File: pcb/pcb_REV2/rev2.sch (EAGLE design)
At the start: 65 parts, among them IC1 PIC24FJ128GA010, IC2 LM1117-XX, IC3 MAX6520, J1 RJ11-6X

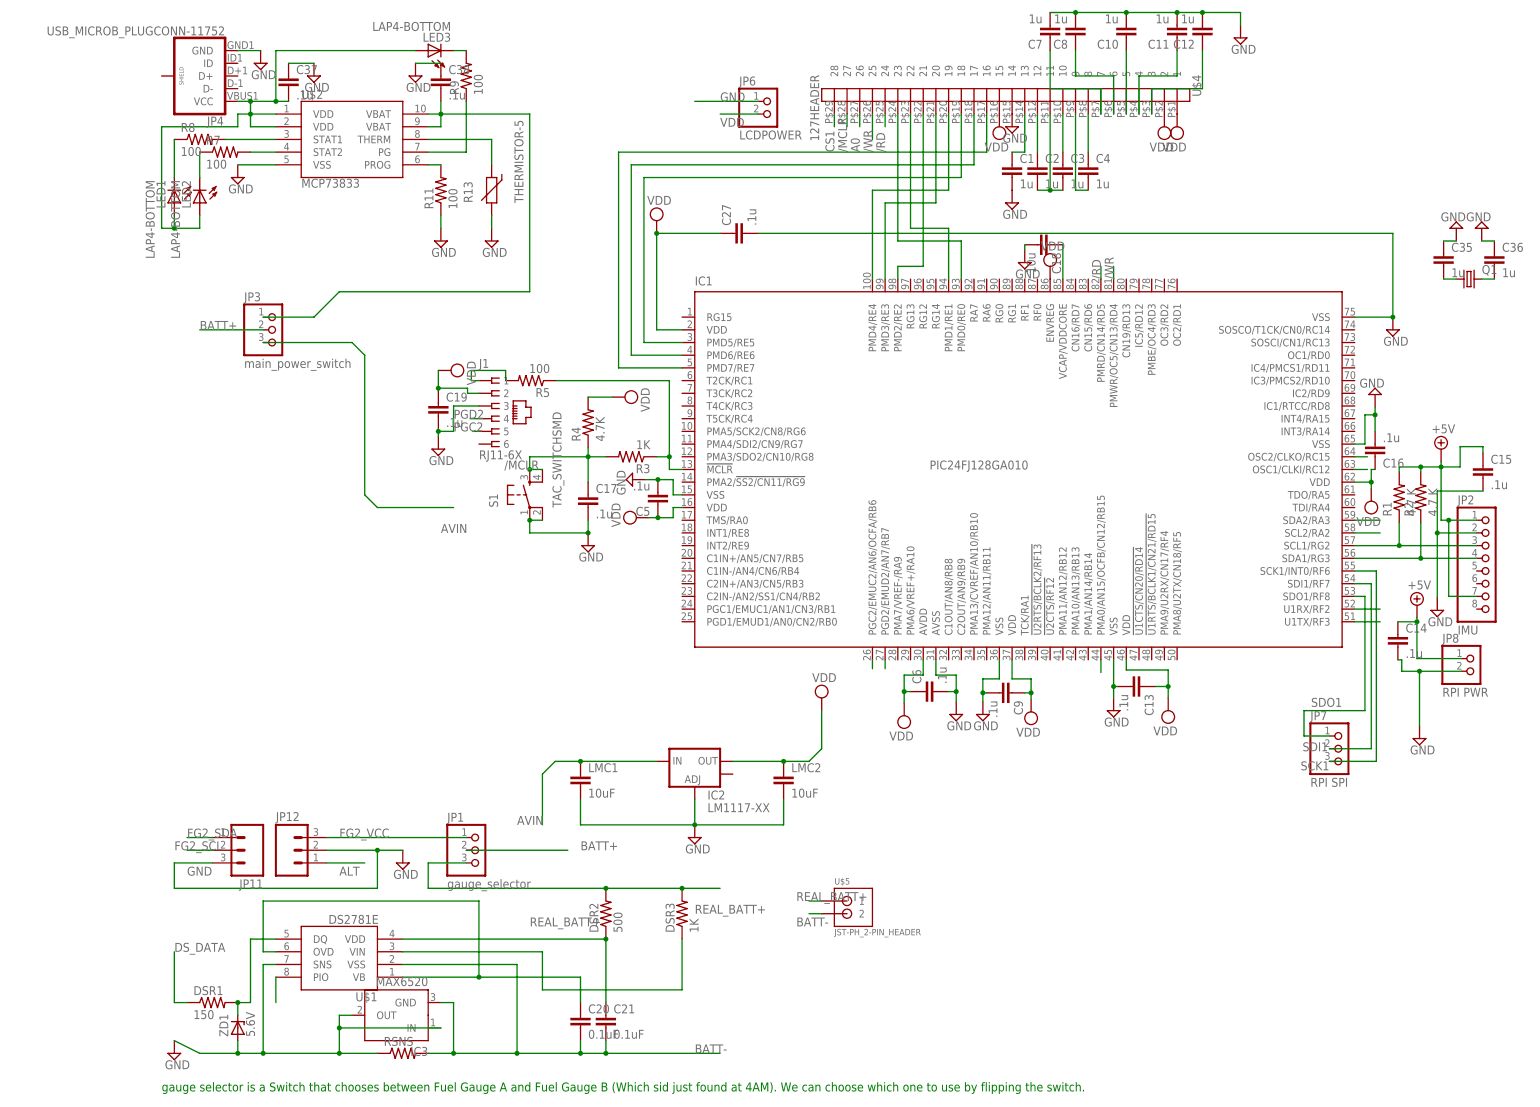
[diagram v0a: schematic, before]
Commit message: go duck
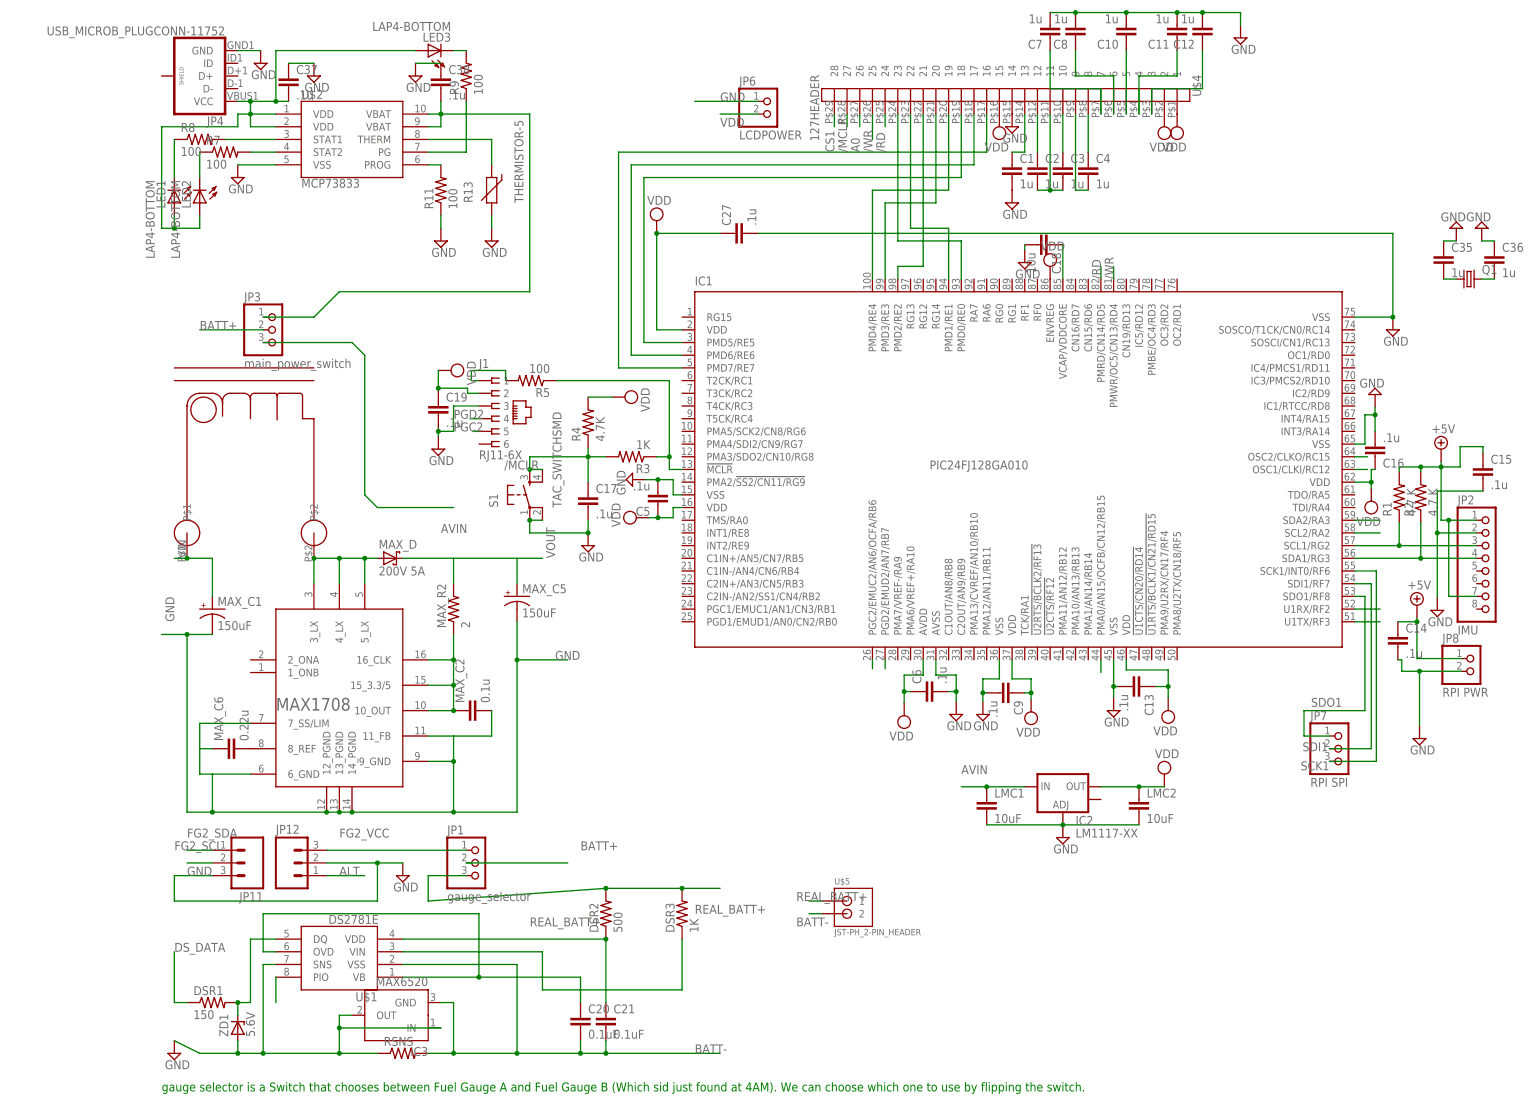
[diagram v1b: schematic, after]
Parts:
- added MAX_C1, MAX_C5: 150uF, adafruit:CPOL-USD/7343-31W
- added MAX_C2: 0.1u, eagle-ltspice:CC1206
- added MAX_C6: 0.22u, eagle-ltspice:CC1206
- added MAX_D: 200V 5A, diode:SCHOTTKY-DIODESMC
- added MAX_R2: 2, adafruit:R-US_R1206
- added U$3: MAX1708, max1708:MAX1708
- added U$6: (no value), fuelgauge:UP2B-2R2-R
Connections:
- new net N$30: MAX_C5.+
- new net N$35: MAX_D.A, U$3.3_LX, U$3.4_LX, U$3.5_LX, U$6.P$2
- new net N$38: MAX_C2.1, MAX_R2.1, U$3.10_OUT, U$3.15_3.3/5, U$3.16_CLK
- new net N$40: MAX_C6.2, U$3.8_REF
- new net VIN: MAX_C1.+, U$6.P$1
- new net VOUT: MAX_D.C, MAX_R2.2
- net GND: now also MAX_C1.-, MAX_C2.2, MAX_C5.-, MAX_C6.1, U$3.11_FB, U$3.12_PGND, U$3.13_PGND, U$3.14_PGND, U$3.6_GND, U$3.7_SS/LIM, U$3.9_GND
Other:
- moved on the sheet: IC2, JP1, JP11, JP12, LMC1, LMC2
